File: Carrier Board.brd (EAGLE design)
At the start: 90.4 x 36.1 mm, 50 parts, among them J4 S2B-PH-SM4-TB(LF)(SN), J5 S2B-PH-SM4-TB(LF)(SN), Q1 MMBT2222A, U1 TMP36GRTZ, U2 TPL5010, U3 MB85RC256, U7 NAND

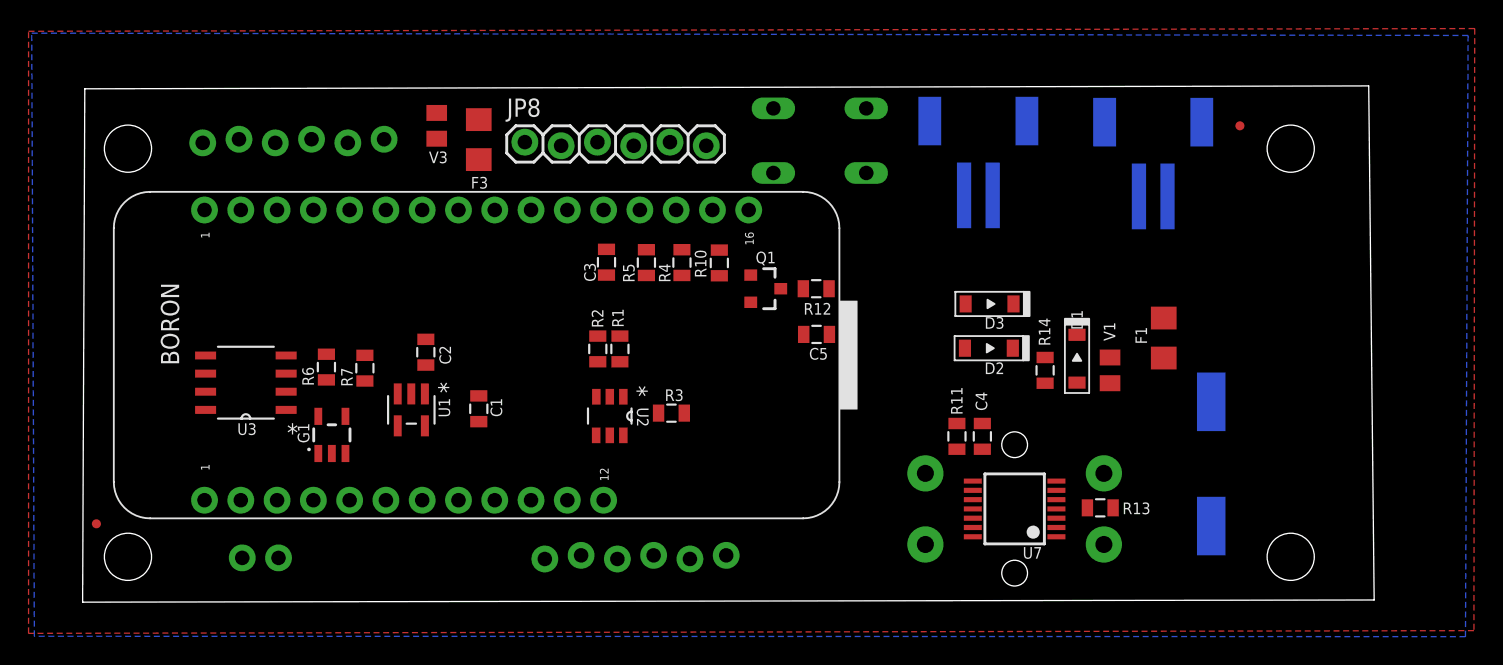
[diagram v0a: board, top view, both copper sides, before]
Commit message: v0.11 - Refining placments
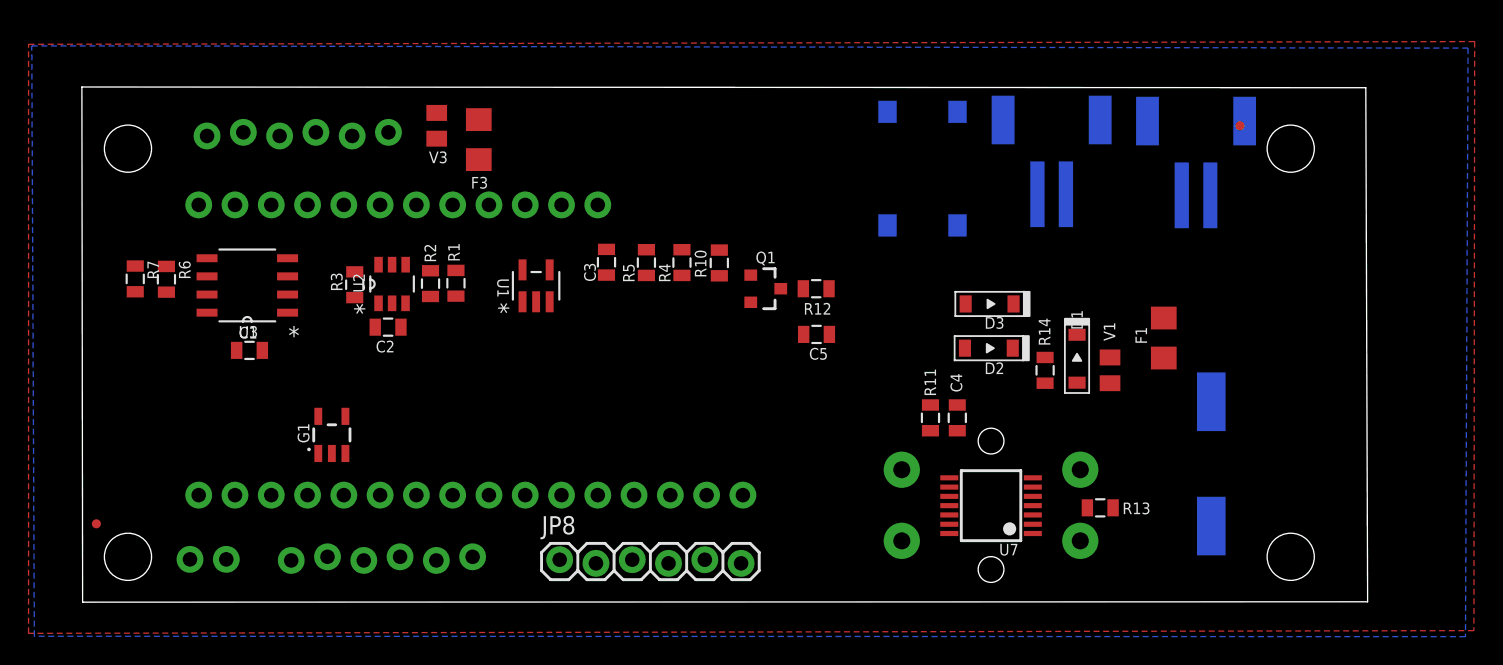
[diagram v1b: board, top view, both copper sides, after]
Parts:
- removed S1: B3F-1070, switch-omron:B3F-10XX
- added SW2: MF-SW-TACT-6MM, MF_Switches:TACT6MM
- moved JP1 37.9 mm to (21.4, 32.9)
- moved JP2 29.9 mm to (14.6, 2.92)
- moved JP8 29.3 mm to (33.4, 2.97)
- moved R3 23.9 mm to (19.1, 22.2), turned to 270 degrees
- moved BORON 22.5 mm to (1.78, 6.22), flipped to the bottom, turned to 90 degrees
- moved U2 17.8 mm to (21.7, 22.3), turned to 90 degrees
- moved R7 17.2 mm to (3.68, 22.6), turned to 270 degrees
- moved C1 16.6 mm to (11.7, 17.6), turned to 0 degrees
- moved R6 12.8 mm to (5.87, 22.6), turned to 270 degrees
- moved R2 12.6 mm to (24.4, 22.3)
- moved R1 12.4 mm to (26.1, 22.3)
- moved U1 12.3 mm to (31.8, 22.1), turned to 90 degrees
- moved U3 6.81 mm to (11.5, 22.2)
- moved J5 5.13 mm to (67.8, 32.3)
- moved J3 3.66 mm to (10.1, 3.00)
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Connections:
- removed net WKP: U2.5
- net GND: now also SW2.P$3, SW2.P$4; no longer S1.3, S1.4
- net N$4: now also SW2.P$1, SW2.P$2; no longer S1.1, S1.2
- net WAKE: now also U2.5
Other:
- board size 90.4 x 36.1 mm -> 90 x 36.1 mm
